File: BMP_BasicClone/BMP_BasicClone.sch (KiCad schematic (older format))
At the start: 53 parts, among them J1 BARREL_JACK, Q1 MMBT3904, Q2 MMBT3904, Q3 MMBT3904, Q4 MMBT3904

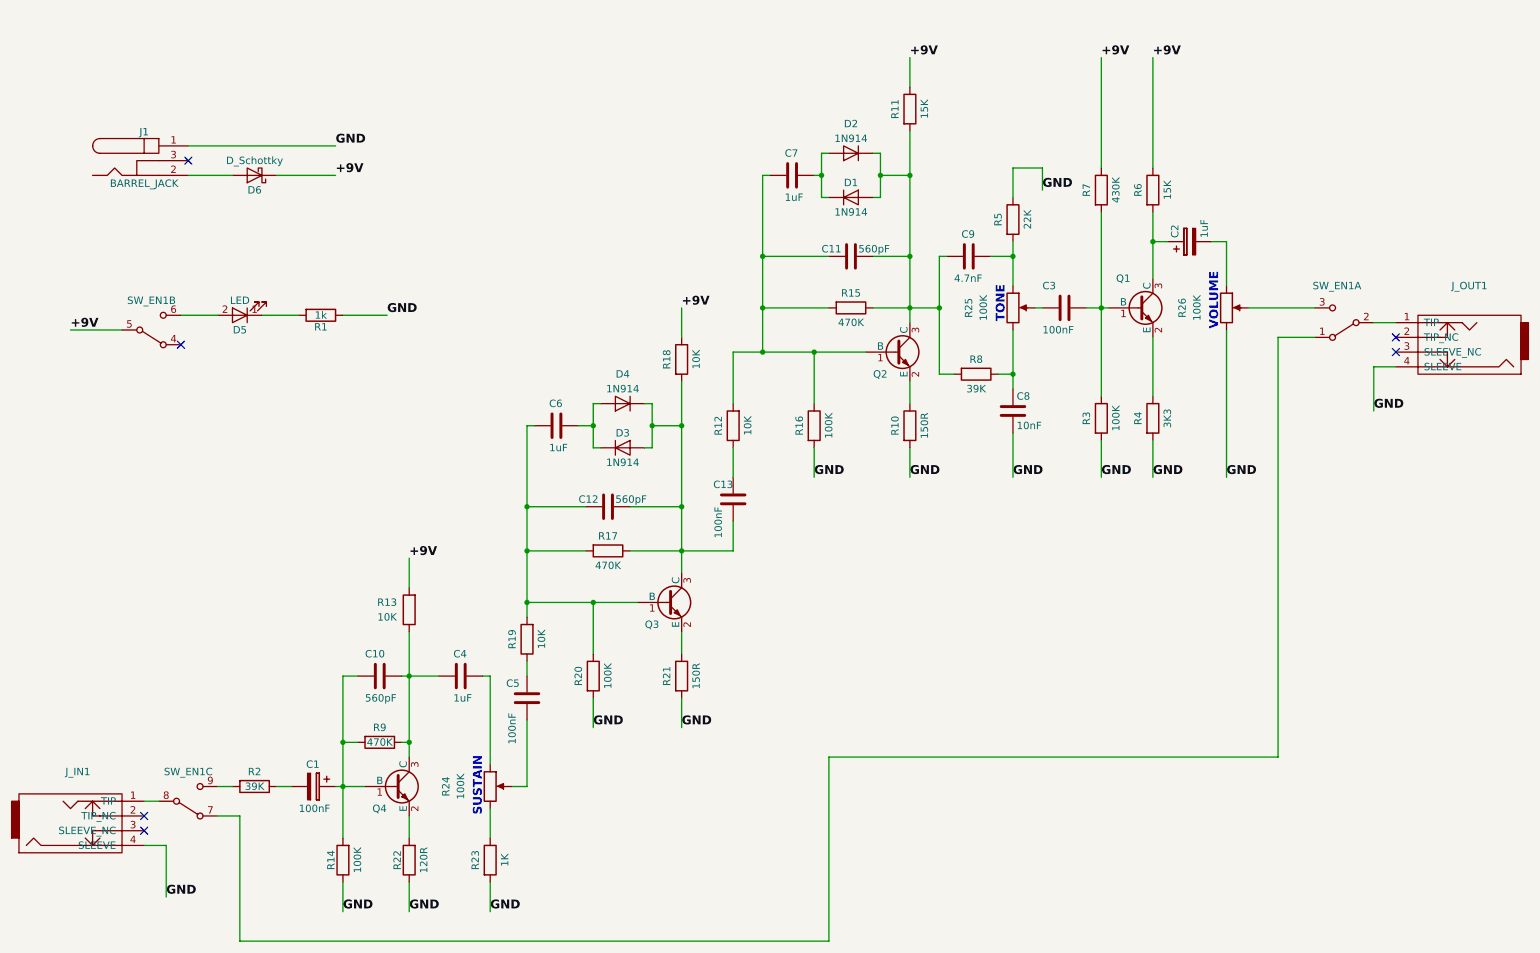
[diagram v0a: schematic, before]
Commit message: update
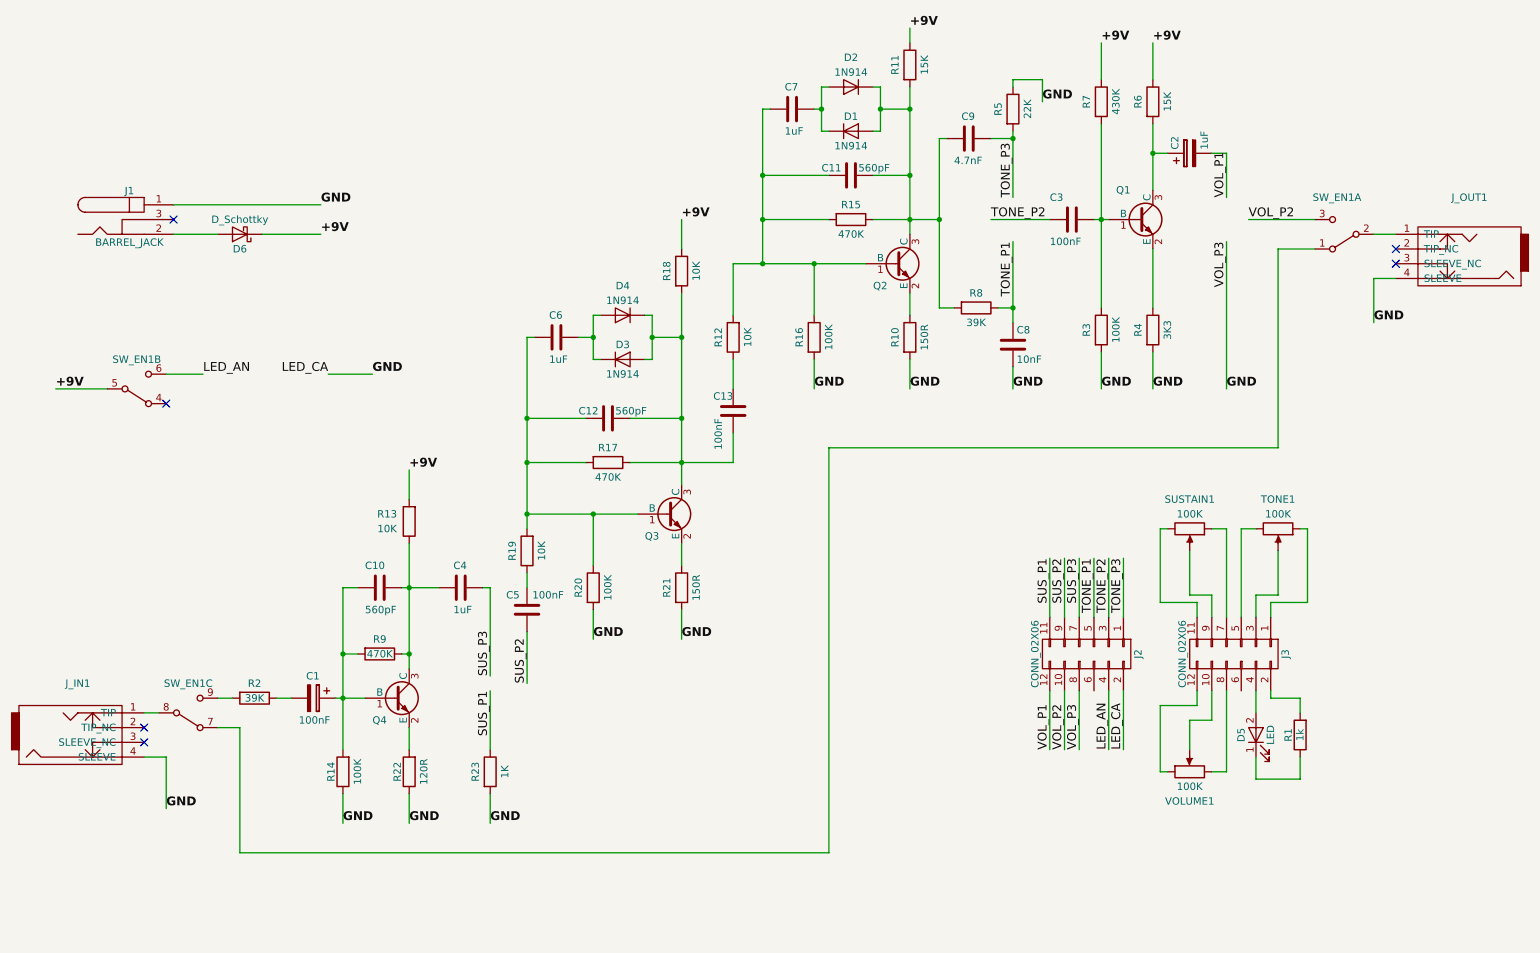
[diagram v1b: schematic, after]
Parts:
- removed R24, R25, R26: 100K, Potentiometers:Potentiometer_Bourns_PTV09A-1_Horizontal, symbol POT
- added J2, J3: CONN_02X06, Pin_Headers:Pin_Header_Straight_2x06_Pitch2.54mm, symbol CONN_02X06
- added SUSTAIN1, TONE1, VOLUME1: 100K, Potentiometers:Potentiometer_Bourns_PTV09A-1_Horizontal, symbol POT
- C1, C10, C11, C12, C13, C2, C3, C4, C5, C6, C7, C8, C9: footprint Capacitors_SMD:C_0402_NoSilk -> Capacitors_SMD:C_0805
- D1, D2, D3, D4, D6: footprint Diodes_SMD:D_SOD-323_HandSoldering -> Diodes_SMD:D_SOD-523
- R1, R10, R11, R12, R13, R14, R15, R16, R17, R18, R19, R2, R20, R21, R22, R23, R3, R4, R5, R6, R7, R8, R9: footprint Resistors_SMD:R_0402_NoSilk -> Resistors_SMD:R_0805
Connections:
- net GND: now also J2.2 (P2), J2.8 (P8); no longer R1.1
- net SUS_P3: now reaches C4.1
- net SUS_P3: now also J2.7 (P7)
- net SUS_P2: now reaches C5.1
- net SUS_P2: now also J2.9 (P9)
- net SUS_P1: now reaches R23.1
- net SUS_P1: now also J2.11 (P11)
- net TONE_P3: now reaches C9.1, R5.2
- net TONE_P3: now also J2.1 (P1)
- net TONE_P1: now reaches C8.1, R8.1
- net TONE_P1: now also J2.5 (P5)
- net TONE_P2: now reaches C3.2
- net TONE_P2: now also J2.3 (P3)
- net VOL_P1: now reaches C2.2
- net VOL_P1: now also J2.12 (P12)
- net VOL_P2: now reaches SW_EN1.3 (C)
- net VOL_P2: now also J2.10 (P10)
- net at D5.2 (A): now also J3.4 (P4); no longer SW_EN1.6 (C)
- net at D5.1 (K): now also R1.1; no longer R1.2
- new net: J3.2 (P2), R1.2
- new net: J3.1 (P1), TONE1.1
- new net: J3.10 (P10), VOLUME1.2
- new net: J3.11 (P11), SUSTAIN1.3
- new net: J3.12 (P12), VOLUME1.1
- new net: J3.3 (P3), TONE1.2
- new net: J3.5 (P5), TONE1.3
- new net: J3.7 (P7), SUSTAIN1.1
- new net: J3.8 (P8), VOLUME1.3
- new net: J3.9 (P9), SUSTAIN1.2
- new net LED_AN: J2.4 (P4), SW_EN1.6 (C)
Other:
- note removed: "SUSTAIN"
- note removed: "TONE"
- note removed: "VOLUME"
- moved on the sheet: C1, C10, C11, C12, C13, C2, C3, C4, C5, C6, C7, C8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
